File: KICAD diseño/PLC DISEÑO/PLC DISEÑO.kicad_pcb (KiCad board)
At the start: 2 copper layers, 23 parts, among them J1 Screw_Terminal_2_P5.00mm, J10 Screw_Terminal_3_P5.00mm, J11 Screw_Terminal_2_P5.00mm, J14 Screw_Terminal_6_P5.00mm, J2 Screw_Terminal_4_P5.00mm, J3 Screw_Terminal_2_P5.00mm, J4 Screw_Terminal_2_P5.00mm, J6 Screw_Terminal_3_P5.00mm, J7 Screw_Terminal_2_P5.00mm, J8 Screw_Terminal_2_P5.00mm, J9 Screw_Terminal_4_P5.00mm, U2 AP63203WU

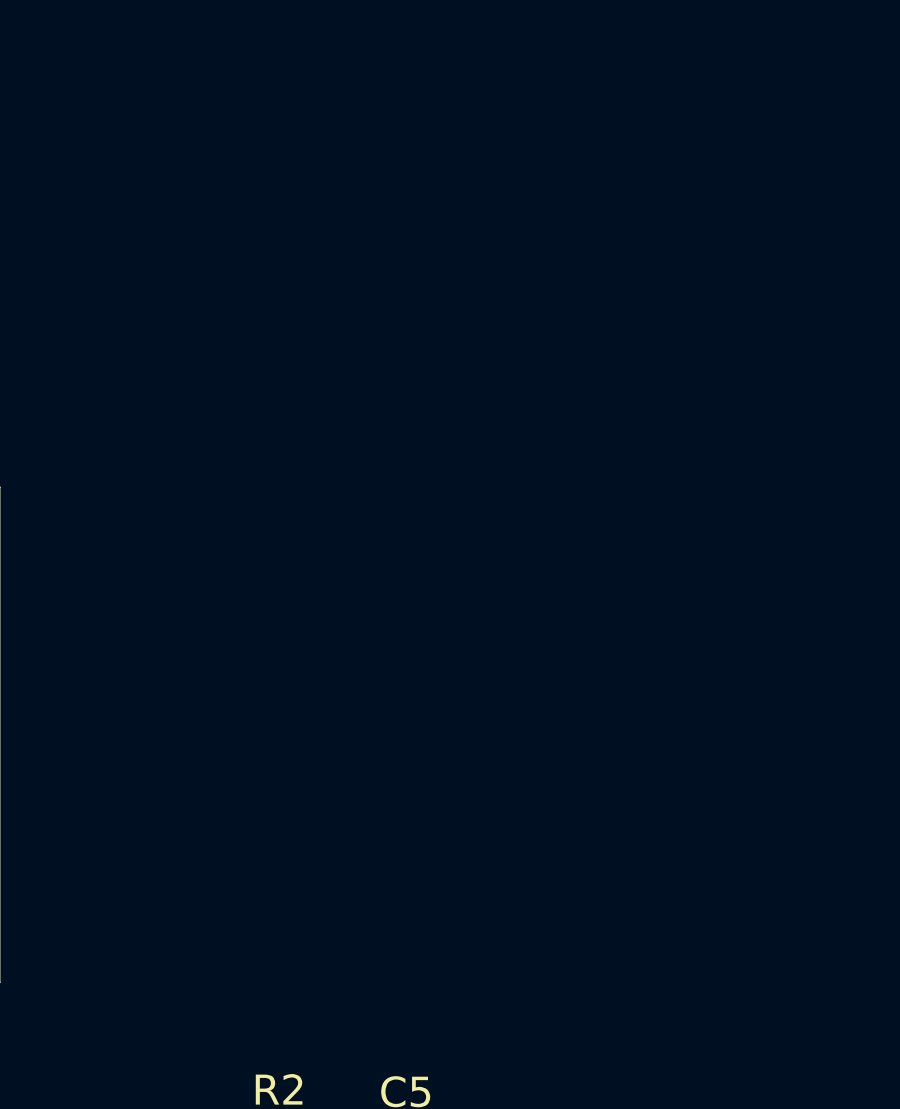
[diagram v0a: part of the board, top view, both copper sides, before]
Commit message: Actualizacion
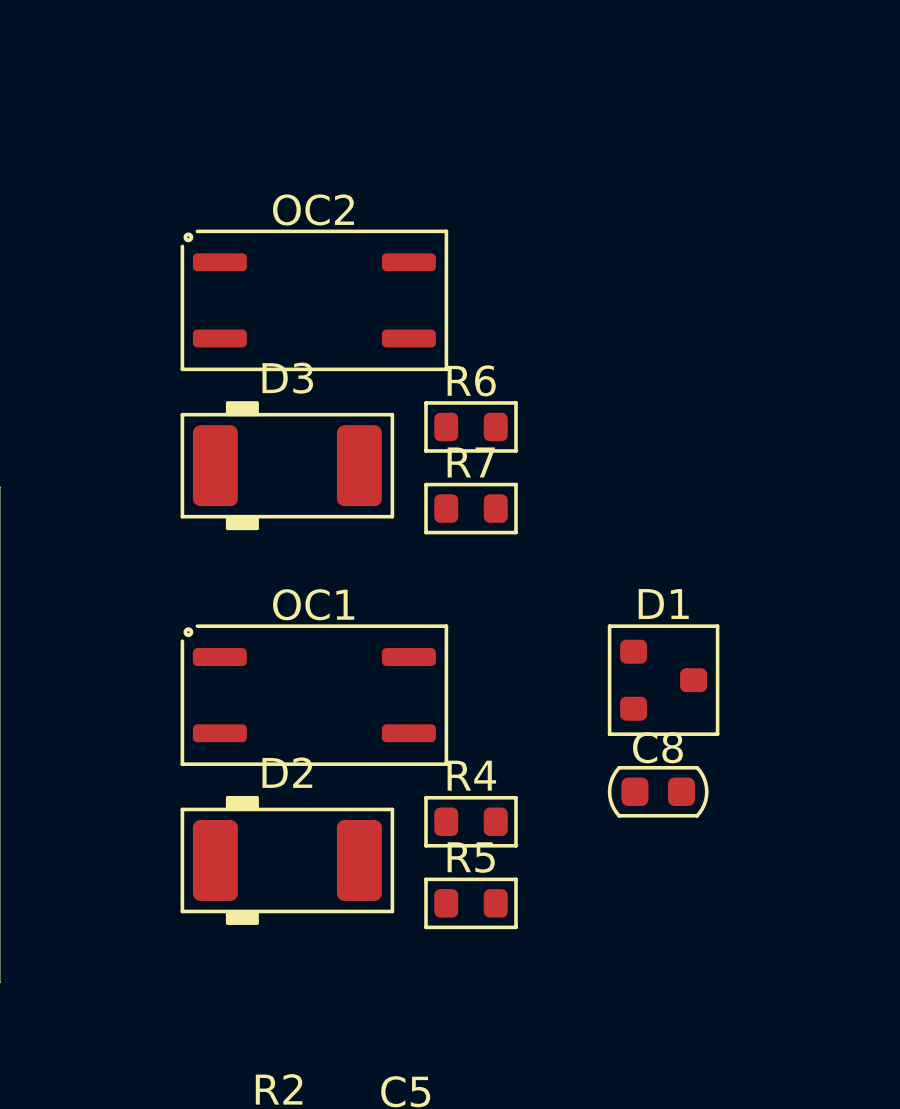
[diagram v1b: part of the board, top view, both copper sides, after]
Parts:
- added C8: C_0603, PCM_Capacitor_SMD_AKL:C_0603_1608Metric, F.Cu at (99.7, 76.2)
- added D1: SM712, PCM_Package_TO_SOT_SMD_AKL:SOT-23, F.Cu at (99.9, 72.5)
- added D2: DL4007, PCM_Diode_SMD_AKL:D_MELF, F.Cu at (87.4, 78.5)
- added D3: DL4007, PCM_Diode_SMD_AKL:D_MELF, F.Cu at (87.4, 65.4)
- added OC1: LTV-357T, PCM_Package_SO_AKL:SO-4_4.4x3.9mm_P2.54mm, F.Cu at (88.3, 73.0)
- added OC2: LTV-357T, PCM_Package_SO_AKL:SO-4_4.4x3.9mm_P2.54mm, F.Cu at (88.3, 59.9)
- added R4: R_0603, PCM_Resistor_SMD_AKL:R_0603_1608Metric, F.Cu at (93.5, 77.2)
- added R5: R_0603, PCM_Resistor_SMD_AKL:R_0603_1608Metric, F.Cu at (93.5, 80.0)
- added R6: R_0603, PCM_Resistor_SMD_AKL:R_0603_1608Metric, F.Cu at (93.5, 64.1)
- added R7: R_0603, PCM_Resistor_SMD_AKL:R_0603_1608Metric, F.Cu at (93.5, 66.8)
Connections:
- net /BOARD_NIRVARA/RFL1_NC renamed /RFL1_NC
- net /BOARD_NIRVARA/RFL2_NC renamed /RFL2_NC
- C2 pad 2: unconnected-(C2-Pad2) -> GND
- C7 pad 1: unconnected-(C7-VCC-Pad1) -> +3.3V
- C7 pad 2: unconnected-(C7-GND-Pad2) -> Net-(C7-GND)
- C7 pad 3: unconnected-(C7-TXD-Pad3) -> /BOARD_NIRVARA/DRIVER_RS485/UART_IN
- C7 pad 4: unconnected-(C7-RXD-Pad4) -> /BOARD_NIRVARA/DRIVER_RS485/UART_OUT
- C7 pad 5: unconnected-(C7-CON-Pad5) -> /BOARD_NIRVARA/DRIVER_RS485/GPIO control
- C7 pad 8: unconnected-(C7-A-Pad8) -> /BOARD_NIRVARA/RS485-B
- C7 pad 9: (no net) -> /BOARD_NIRVARA/RS485-A

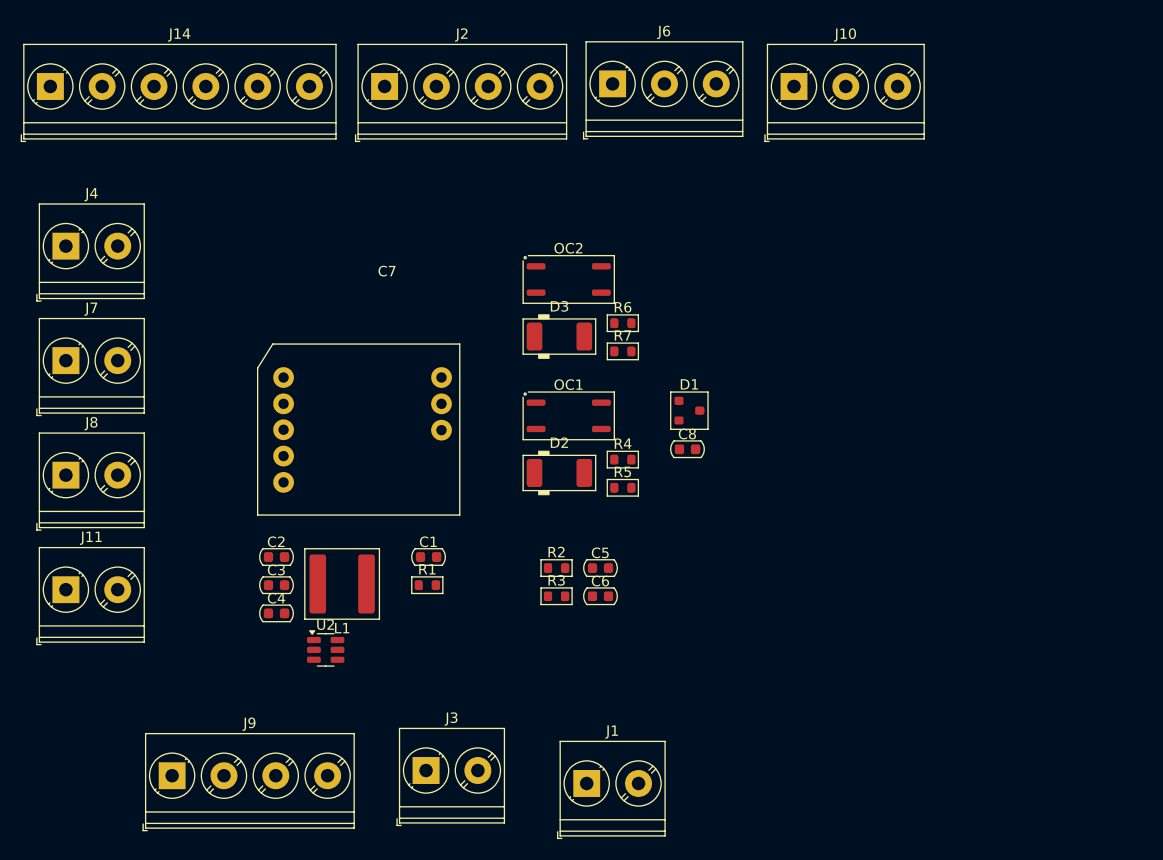
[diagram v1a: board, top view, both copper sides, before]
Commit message: Actualizacion estoy cansado jefe :)
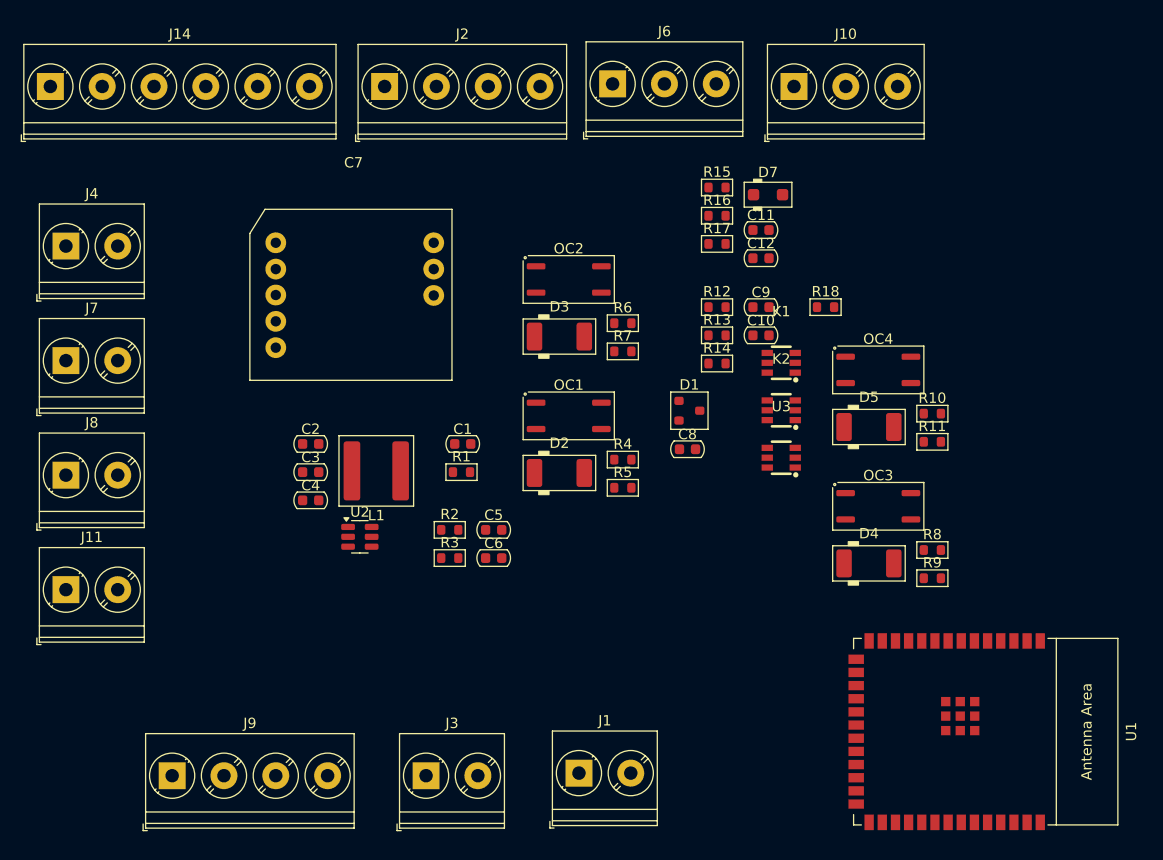
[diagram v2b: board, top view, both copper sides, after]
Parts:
- added C10: C_0603, PCM_Capacitor_SMD_AKL:C_0603_1608Metric, F.Cu at (106.8, 65.3)
- added C11: C_0603, PCM_Capacitor_SMD_AKL:C_0603_1608Metric, F.Cu at (106.8, 55.1)
- added C12: C_0603, PCM_Capacitor_SMD_AKL:C_0603_1608Metric, F.Cu at (106.8, 57.8)
- added C9: C_0603, PCM_Capacitor_SMD_AKL:C_0603_1608Metric, F.Cu at (106.8, 62.5)
- added D4: DL4007, PCM_Diode_SMD_AKL:D_MELF, F.Cu at (117.2, 87.3)
- added D5: DL4007, PCM_Diode_SMD_AKL:D_MELF, F.Cu at (117.2, 74.1)
- added D7: SMF24A, PCM_Diode_SMD_AKL:D_SOD-123F, F.Cu at (107.5, 51.7)
- added K1: SRA-24VDC-CL, cris:SOT-23-6_L2.9-W1.6-P0.95-LS2.8-BR, F.Cu at (108.8, 67.9)
- added K2: SRA-24VDC-CL, cris:SOT-23-6_L2.9-W1.6-P0.95-LS2.8-BR, F.Cu at (108.8, 72.5)
- added OC3: LTV-357T, PCM_Package_SO_AKL:SO-4_4.4x3.9mm_P2.54mm, F.Cu at (118.1, 81.8)
- added OC4: LTV-357T, PCM_Package_SO_AKL:SO-4_4.4x3.9mm_P2.54mm, F.Cu at (118.1, 68.6)
- added R10: R_0603, PCM_Resistor_SMD_AKL:R_0603_1608Metric, F.Cu at (123.3, 72.8)
- added R11: R_0603, PCM_Resistor_SMD_AKL:R_0603_1608Metric, F.Cu at (123.3, 75.5)
- added R12: R_0603, PCM_Resistor_SMD_AKL:R_0603_1608Metric, F.Cu at (102.6, 62.5)
- added R13: R_0603, PCM_Resistor_SMD_AKL:R_0603_1608Metric, F.Cu at (102.6, 65.3)
- added R14: R_0603, PCM_Resistor_SMD_AKL:R_0603_1608Metric, F.Cu at (102.6, 68.0)
- added R15: R_0603, PCM_Resistor_SMD_AKL:R_0603_1608Metric, F.Cu at (102.6, 51.0)
- added R16: R_0603, PCM_Resistor_SMD_AKL:R_0603_1608Metric, F.Cu at (102.6, 53.7)
- added R17: R_0603, PCM_Resistor_SMD_AKL:R_0603_1608Metric, F.Cu at (102.6, 56.4)
- added R18: R_0603, PCM_Resistor_SMD_AKL:R_0603_1608Metric, F.Cu at (113.0, 62.5)
- added R8: R_0603, PCM_Resistor_SMD_AKL:R_0603_1608Metric, F.Cu at (123.3, 86.0)
- added R9: R_0603, PCM_Resistor_SMD_AKL:R_0603_1608Metric, F.Cu at (123.3, 88.7)
- added U1: ESP32-S3-WROOM-1, ESP32-S3-WROM-1:ESP32-S3-WROOM-1, F.Cu at (125.5, 103.5)
- added U3: LK1802, cris:SOT-23-6_L2.9-W1.6-P0.95-LS2.8-BR, F.Cu at (108.8, 77.1)
- moved C7 13.0 mm to (70.0, 46.6)
- moved C4 11.4 mm to (63.4, 81.2)
- moved R1 11.4 mm to (77.9, 78.5)
- moved C1 11.4 mm to (78.0, 75.7)
- moved C2 11.4 mm to (63.4, 75.7)
- moved C3 11.4 mm to (63.4, 78.5)
- moved L1 11.4 mm to (69.7, 78.3)
- moved U2 11.4 mm to (68.1, 84.7)
- moved R2 10.9 mm to (76.8, 84.0)
- moved R3 10.9 mm to (76.8, 86.7)
- moved C5 10.9 mm to (81.0, 84.0)
- moved C6 10.9 mm to (81.0, 86.8)
- moved J1 1.25 mm to (89.2, 107.5)
- moved J3 0.50 mm to (74.5, 107.8)
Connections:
- net /BOARD_NIRVARA/INPUT_NPN/NPN_input renamed /BOARD_NIRVARA/INPUT_NPN/NPN_input_1
- net /BOARD_NIRVARA/INPUT_PNP/PNP_input renamed /BOARD_NIRVARA/INPUT_PNP/PNP_input_1
- D2 pad 2: /BOARD_NIRVARA/NPN_IN_1 -> GND
- D3 pad 2: /BOARD_NIRVARA/PNP_IN_2 -> GND
- OC1 pad 2: /BOARD_NIRVARA/NPN_IN_1 -> GND
- OC2 pad 2: /BOARD_NIRVARA/PNP_IN_2 -> GND
- R4 pad 1: /BOARD_NIRVARA/NPN_IN_2 -> /BOARD_NIRVARA/NPN_IN_1
